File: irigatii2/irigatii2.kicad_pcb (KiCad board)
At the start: 2 copper layers, 100 x 100 mm, 130 parts, among them IC1 MIC3172YN, IC2 PCA9575PW2,118, J1 Conn_01x02, J2 Conn_01x05, J5 valve, J6 valve, J7 valve, J8 valve, J9 valve, Q11 PMOS, Q12 PMOS, Q13 PMOS, Q14 PMOS, Q15 NMOS, Q16 NMOS, Q17 NMOS, Q18 NMOS, Q19 NMOS, Q20 NMOS, Q21 NMOS, Q22 NMOS, Q23 PMOS, Q24 PMOS, Q25 PMOS, Q26 PMOS, Q27 NMOS, Q28 NMOS, Q29 NMOS, Q30 NMOS, Q31 NMOS, Q32 NMOS, Q33 NMOS, Q34 NMOS, Q35 PMOS, Q36 PMOS, Q37 NMOS, Q38 NMOS, T1 Transformer_1P_1S, U1 NJM2114, U2 TL431LP

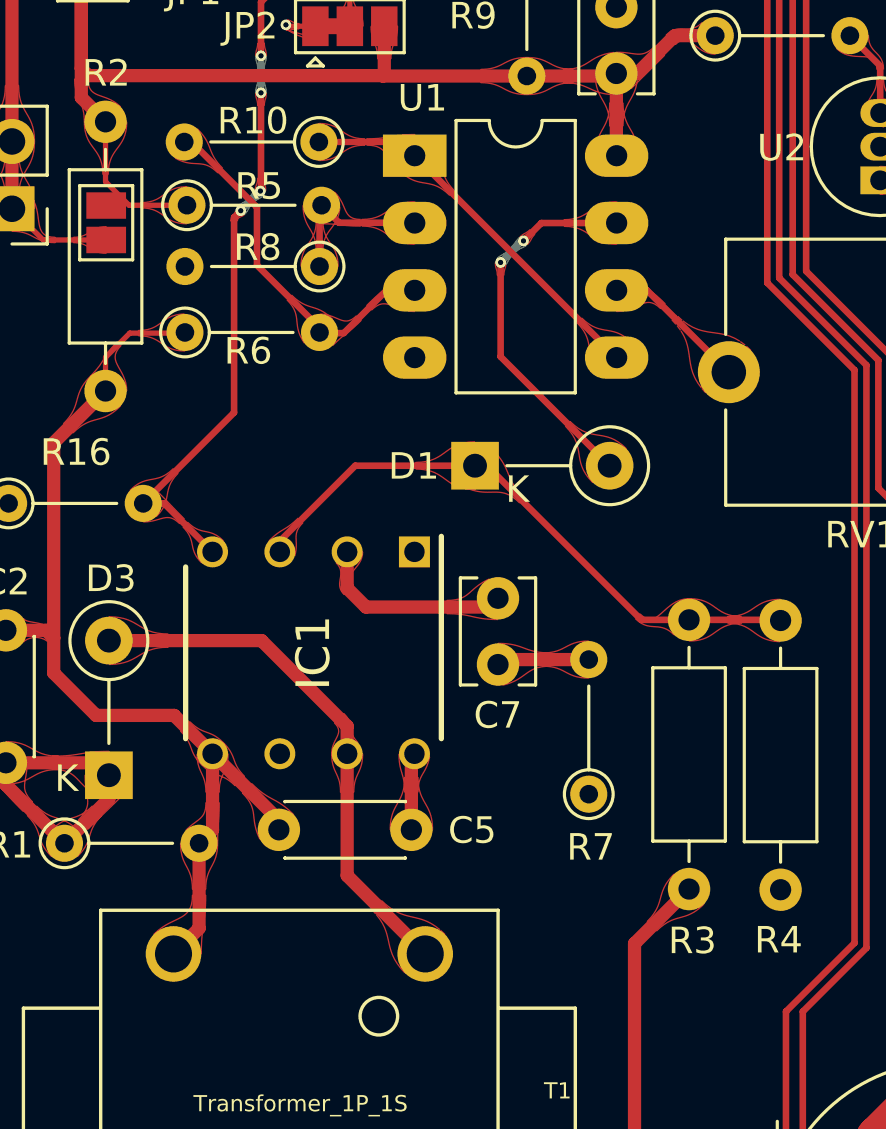
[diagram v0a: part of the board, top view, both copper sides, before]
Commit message: h
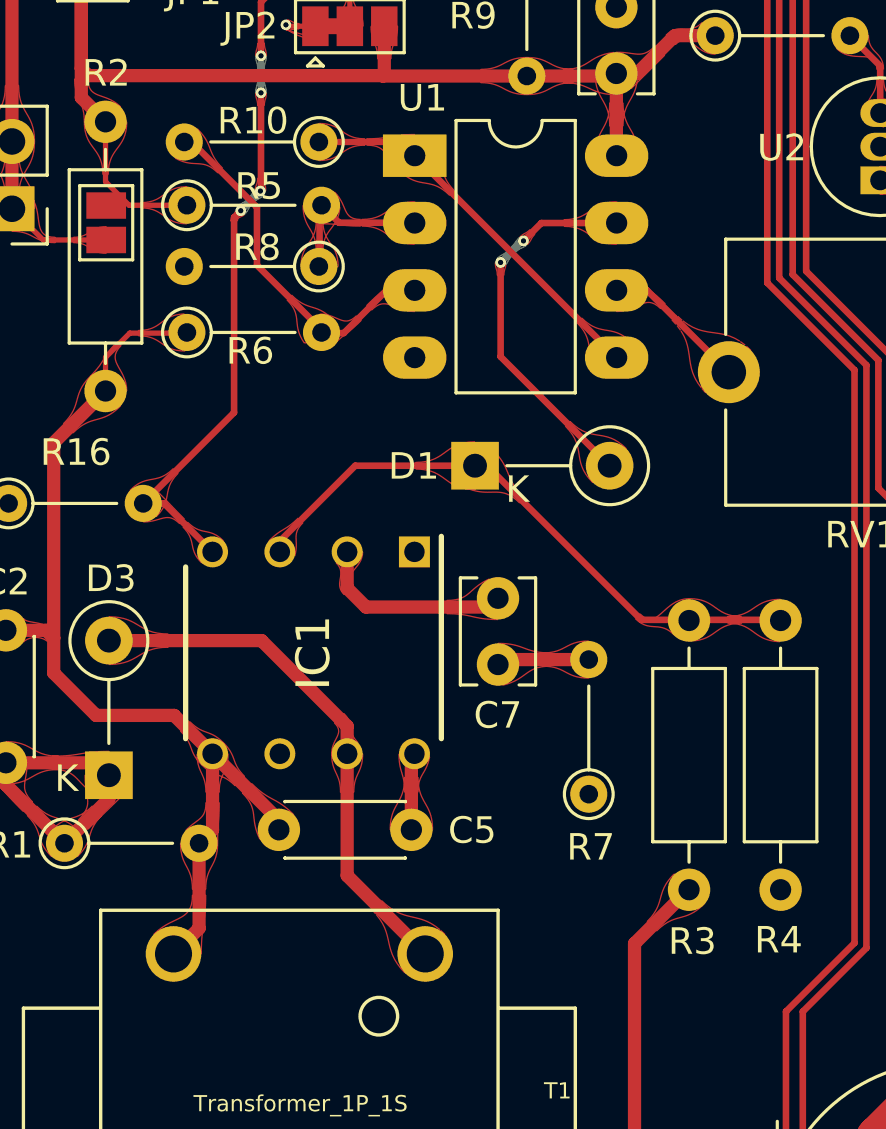
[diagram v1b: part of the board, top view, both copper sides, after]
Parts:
- moved R6 0.07 mm to (36.4, 116.6)
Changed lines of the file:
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@@
   )
   (footprint "Resistor_THT:R_Axial_DIN0204_L3.6mm_D1.6mm_P5.08mm_Vertical" (layer "F.Cu")
-    (at 36.449 111.8108)
+    (at 36.4474 111.8108)
     (descr "Resistor, Axial_DIN0204 series, Axial, Vertical, pin pitch=5.08mm, 0.167W, length*diameter=3.6*1.6mm^2, http://cdn-reichelt.de/documents/datenblatt/B400/1_4W%23YAG.pdf")
     (tags "Resistor Axial_DIN0204 series Axial Vertical pin pitch 5.08mm 0.167W length 3.6mm diameter 1.6mm")
@@
   )
   (footprint "Resistor_THT:R_Axial_DIN0204_L3.6mm_D1.6mm_P5.08mm_Vertical" (layer "F.Cu")
-    (at 41.4528 114.1222 180)
+    (at 41.4274 114.1222 180)
     (descr "Resistor, Axial_DIN0204 series, Axial, Vertical, pin pitch=5.08mm, 0.167W, length*diameter=3.6*1.6mm^2, http://cdn-reichelt.de/documents/datenblatt/B400/1_4W%23YAG.pdf")
     (tags "Resistor Axial_DIN0204 series Axial Vertical pin pitch 5.08mm 0.167W length 3.6mm diameter 1.6mm")
@@
   )
   (footprint "Resistor_THT:R_Axial_DIN0207_L6.3mm_D2.5mm_P10.16mm_Horizontal" (layer "F.Cu")
-    (at 55.3974 127.4572 -90)
+    (at 55.3974 127.4826 -90)
     (descr "Resistor, Axial_DIN0207 series, Axial, Horizontal, pin pitch=10.16mm, 0.25W = 1/4W, length*diameter=6.3*2.5mm^2, http://cdn-reichelt.de/documents/datenblatt/B400/1_4W%23YAG.pdf")
     (tags "Resistor Axial_DIN0207 series Axial Horizontal pin pitch 10.16mm 0.25W = 1/4W length 6.3mm diameter 2.5mm")
@@
   )
   (footprint "Resistor_THT:R_Axial_DIN0204_L3.6mm_D1.6mm_P5.08mm_Vertical" (layer "F.Cu")
-    (at 36.3728 116.6114)
+    (at 36.4474 116.6114)
     (descr "Resistor, Axial_DIN0204 series, Axial, Vertical, pin pitch=5.08mm, 0.167W, length*diameter=3.6*1.6mm^2, http://cdn-reichelt.de/documents/datenblatt/B400/1_4W%23YAG.pdf")
     (tags "Resistor Axial_DIN0204 series Axial Vertical pin pitch 5.08mm 0.167W length 3.6mm diameter 1.6mm")
